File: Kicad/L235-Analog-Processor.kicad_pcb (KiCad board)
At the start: 2 copper layers, 110 x 110 mm, 304 parts, among them IC2 AD633ARZ-RL, J1 Input A, J10 Half Wave A + -B, J11 Inverted Out B, J12 CV Select, J13 CV Select, J14 Conn_01x12_Pin, J15 Inverted Out A, J16 Full-Wave Rectifier A, J17 Half-Wave Rectifier A, J18 √(A²+B²), J19 Conn_01x12_Socket, J2 Input B, J3 Function IN, J4 ( 10A / |B| ) / ( A * B / 10 ), J5 Output F(x), J6 Power, J7 Full-Wave Rectifier B, J8 A - B, J9 Negative Half-Wave Rectifier B, U1 TL082, U10 TL082, U11 TL082, U12 TL082, U13 TL084, U14 RC4580, U15 TL082, U17 TL082, U18 LM4040DBZ-10, U19 74HC148, U2 TL082, U20 LM339, U21 LM339, U22 DG4051E, U23 DG4051E, U24 DG4051E, U25 DG4051E, U26 DG4051E, U27 74LS151, U28 DG4051E, U29 LM339, U3 TL082, U30 LM339, U31 74HC148, U32 DG4051E, U33 DG4051E, U34 DG4051E, U35 DG4051E, U36 LM78M05_TO252, U37 TL082, U4 TL082, U5 TL082, U6 TL082, U7 TL082, U8 TL082, U9 TL082

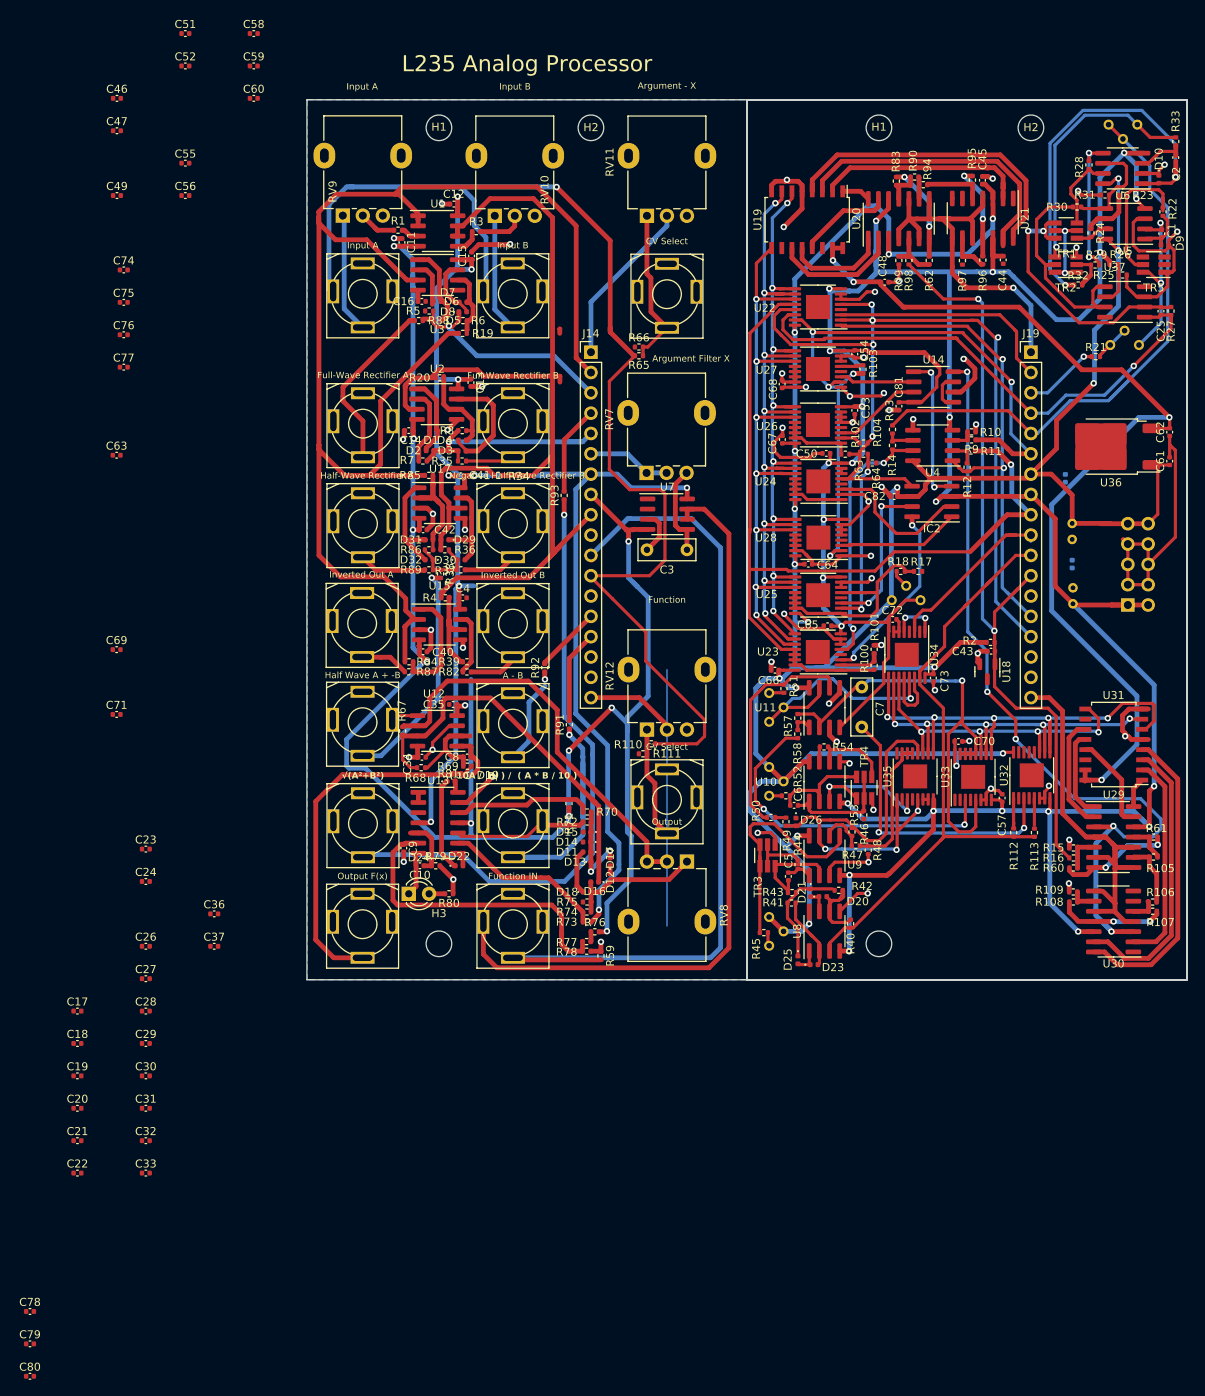
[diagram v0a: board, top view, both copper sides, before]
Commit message: All components routed
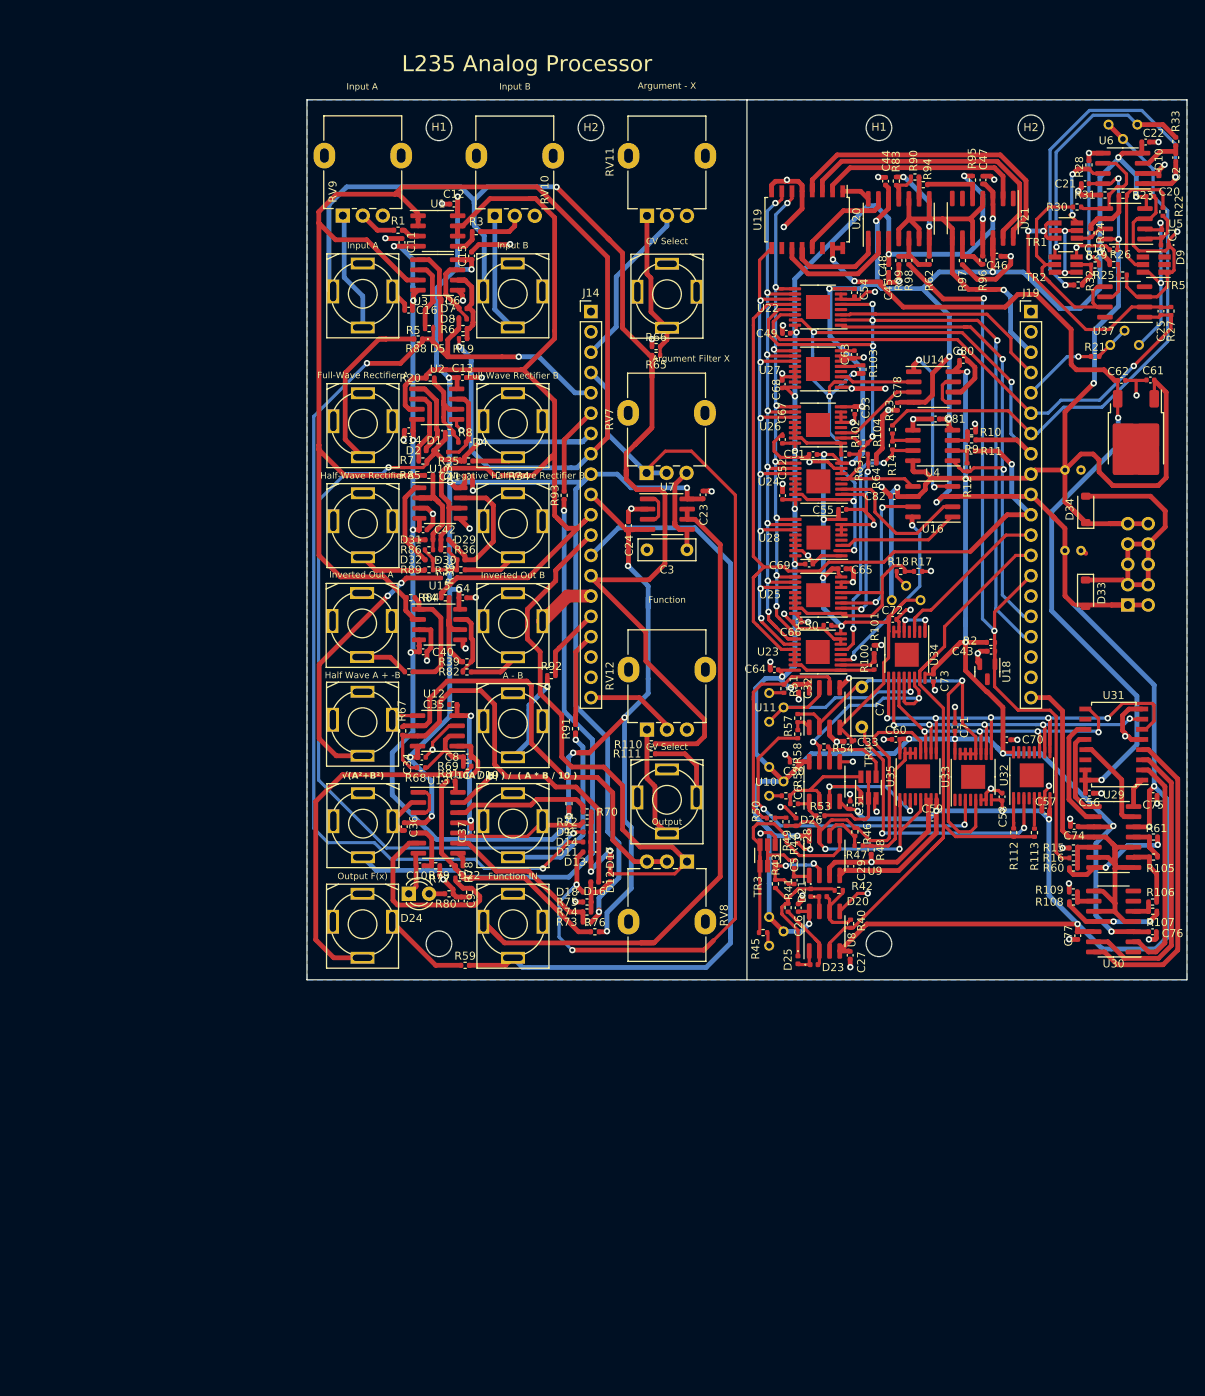
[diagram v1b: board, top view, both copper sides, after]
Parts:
- removed C17, C18, C79: 100nF, Capacitor_SMD:C_0402_1005Metric
- removed D27, D28: 1N5819, Diode_SMD:D_0402_1005Metric
- removed IC2: AD633ARZ-RL, Package_SO:SOIC-8_3.9x4.9mm_P1.27mm
- added D33: 1N5819HW, Diode_SMD:D_SOD-123, F.Cu at (399.8, 61.7)
- added D34: 1N5819HW, Diode_SMD:D_SOD-123, F.Cu at (399.9, 51.2)
- added U16: AD633ARZ-RL, Package_SO:SOIC-8_3.9x4.9mm_P1.27mm, F.Cu at (380.7, 50.2)
- J14: value Conn_01x12_Pin -> Conn_01x20_Pin; footprint Connector_PinHeader_2.54mm:PinHeader_1x18_P2.54mm_Vertical -> Connector_PinHeader_2.54mm:PinHeader_1x20_P2.54mm_Vertical
- J19: value Conn_01x12_Socket -> Conn_01x20_Socket; footprint Connector_PinHeader_2.54mm:PinHeader_1x18_P2.54mm_Vertical -> Connector_PinHeader_2.54mm:PinHeader_1x20_P2.54mm_Vertical
- moved C22 185.6 mm to (407.3, 5.28), turned to 180 degrees
- moved C20 176.0 mm to (407.9, 12.1), turned to 180 degrees
- moved C21 173.7 mm to (399.8, 10.5), turned to 180 degrees
- moved C80 172.4 mm to (384.5, 32.6)
- moved C19 165.6 mm to (403.3, 18.7), turned to 180 degrees
- moved C78 156.7 mm to (376.3, 38.3), turned to 90 degrees
- moved C76 148.7 mm to (408.2, 104.0)
- moved C75 142.7 mm to (408.3, 87.0), turned to 180 degrees
- moved C77 138.8 mm to (398.9, 104.5), turned to 90 degrees
- moved C74 137.7 mm to (398.4, 90.8), turned to 180 degrees
- moved C56 135.5 mm to (400.3, 86.7), turned to 180 degrees
- moved C58 133.6 mm to (389.4, 87.1), turned to -90 degrees
- moved C59 126.6 mm to (380.7, 89.8)
- moved C60 113.4 mm to (376.1, 80.0)
- moved C46 111.8 mm to (388.8, 19.6), turned to 180 degrees
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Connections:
- C74 pad 1: Net-(U14C-V+) -> +12V
- C76 pad 1: Net-(U14C-V+) -> +12V
- C80 pad 1: Net-(U14C-V+) -> +12V
- J14 pad 1: CV_SELECT -> unconnected-(J14-Pin_1-Pad1)
- J14 pad 10: Function Out -> -12V
- J14 pad 11: <X> -> B
- J14 pad 12: 10V REF -> Function Out
- J14 pad 13: GND -> <X>
- J14 pad 14: A - B -> 10V REF
- J14 pad 15: AD534_OUT -> GND
- J14 pad 16: GND -> A - B
- J14 pad 17: GND -> AD534_OUT
- J14 pad 18: CV_FUNCTION -> GND
- J14 pad 2: X -> GND
- J14 pad 3: |A| -> CV_SELECT
- J14 pad 4: √(A²+B²) -> X
- J14 pad 5: |B| -> |A|
- J14 pad 6: A -> √(A²+B²)
- J14 pad 7: +12V -> |B|
- J14 pad 8: -12V -> A
- J14 pad 9: B -> +12V
- J19 pad 1: CV_SELECT -> unconnected-(J19-Pin_1-Pad1)
- J19 pad 10: Function Out -> -12V
- J19 pad 11: <X> -> B
- J19 pad 12: 10V REF -> Function Out
- J19 pad 13: GND -> <X>
- J19 pad 14: A - B -> 10V REF
- J19 pad 15: AD534_OUT -> GND
- J19 pad 16: GND -> A - B
- J19 pad 17: GND -> AD534_OUT
- J19 pad 18: CV_FUNCTION -> GND
- J19 pad 2: X -> GND
- J19 pad 3: |A| -> CV_SELECT
- J19 pad 4: √(A²+B²) -> X
- J19 pad 5: |B| -> |A|
- J19 pad 6: A -> √(A²+B²)
- J19 pad 7: +12V -> |B|
- J19 pad 8: -12V -> A
- J19 pad 9: B -> +12V
- U13 pad 1: (no net) -> Net-(U13A-+)
- U13 pad 2: (no net) -> GND
- U13 pad 3: (no net) -> Net-(U13A-+)
- U14 pad 8: Net-(U14C-V+) -> +12V
- U29 pad 3: Net-(U14C-V+) -> +12V
- U30 pad 3: Net-(U14C-V+) -> +12V
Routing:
- net GND: track 291.9 -> 411.6 mm, vias 57 -> 83
- net |A|: track 38.7 -> 148.0 mm, vias 2 -> 4
- net X: track 45.5 -> 153.0 mm, vias 0 -> 2
- net Net-(U14C-V+): track 103.1 -> 0.00 mm, vias 5 -> 0
- net +12V: track 565.4 -> 663.8 mm, vias 28 -> 33
- net |B|: track 104.5 -> 191.7 mm, vias 1 -> 3
- net Function Out: track 35.5 -> 91.3 mm
- net -12V: track 641.3 -> 670.4 mm, vias 35 -> 34
- net A: track 273.8 -> 296.0 mm, vias 5 -> 7
- net Net-(D19-K): track 12.9 -> 34.7 mm
- net √|x| or X²: track 10.1 -> 26.6 mm, vias 0 -> 2
- net Net-(U13B--): track 39.7 -> 26.9 mm
- net Net-(J4-PadT): track 34.6 -> 23.0 mm
- net Net-(U7B--): track 96.0 -> 86.8 mm
- net B: track 234.6 -> 226.5 mm
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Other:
- board text added: "Version 1.0 Lytrix 2024"
